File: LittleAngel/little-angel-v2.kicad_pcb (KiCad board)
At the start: 2 copper layers, 55.5 x 100 mm, 59 parts, among them J1 IN, J2 V+ GND, J3 V+ GND, J4 OUT, Q1 2N3904, SW1 SW_3PDT, U1 NE5532, U2 L78L05_TO92, U3 PT2399

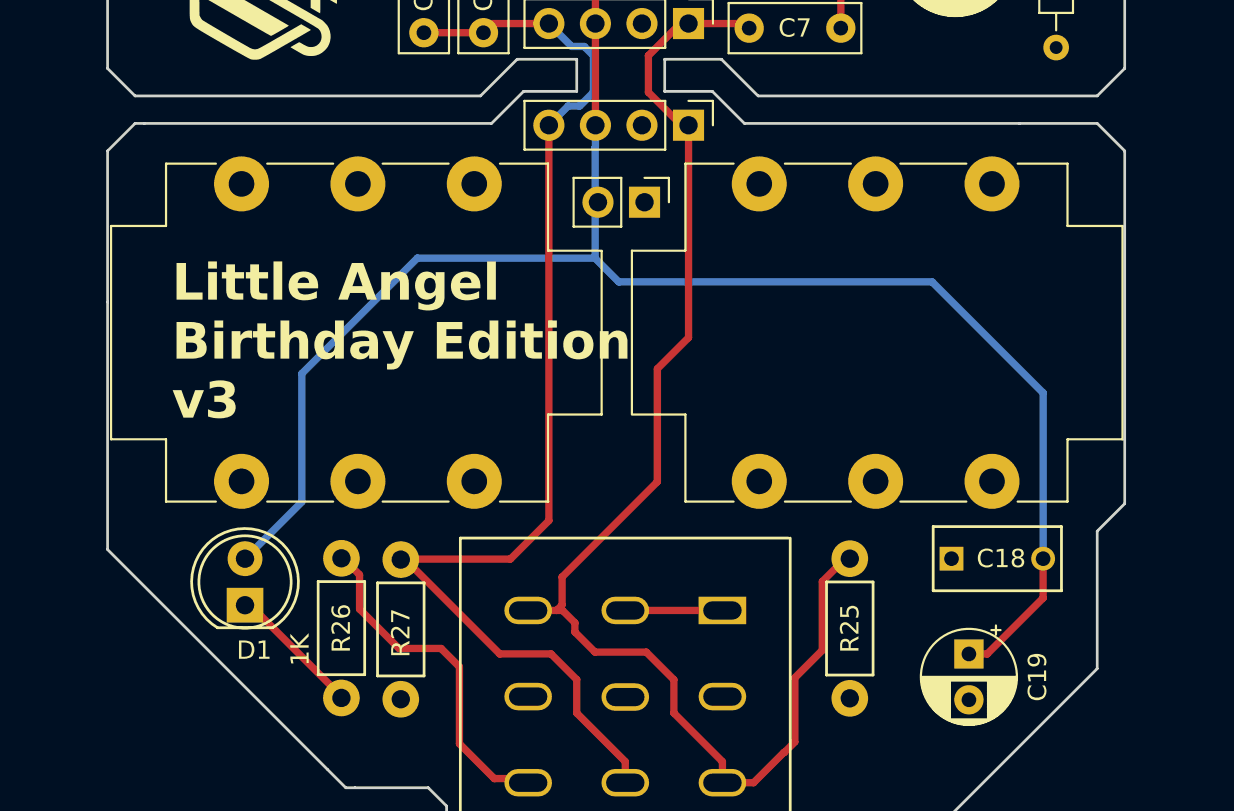
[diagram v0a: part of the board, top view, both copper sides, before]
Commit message: WIP
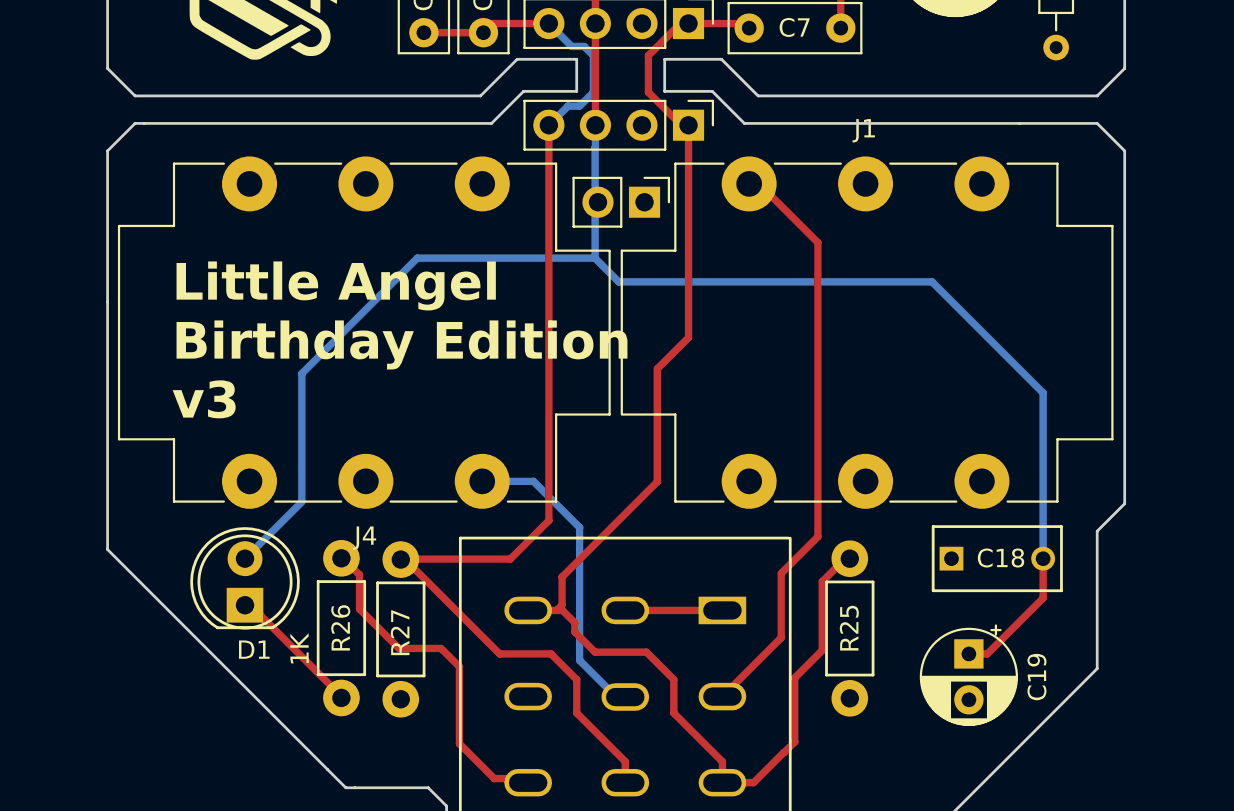
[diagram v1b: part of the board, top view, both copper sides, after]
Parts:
- J1: value IN -> NMJ6HCD2; footprint Pedal-Components:Jack_6.35mm_Neutrik_NMJ6HCD2_Horizontal -> Connector_Audio:Jack_6.35mm_Neutrik_NMJ6HCD2_Horizontal
- J4: value OUT -> NMJ6HCD2; footprint Pedal-Components:Jack_6.35mm_Neutrik_NMJ6HCD2_Horizontal -> Connector_Audio:Jack_6.35mm_Neutrik_NMJ6HCD2_Horizontal
- moved J1 0.55 mm to (150.0, 114.5)
- moved J4 0.44 mm to (135.4, 130.8)
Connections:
- J1 pad R: (no net) -> unconnected-(J1-PadR)
- J1 pad RN: (no net) -> unconnected-(J1-PadRN)
- J1 pad S: (no net) -> GND
- J1 pad SN: (no net) -> unconnected-(J1-PadSN)
- J1 pad T: (no net) -> Net-(SW1A-B)
- J1 pad TN: (no net) -> GND
- J4 pad R: (no net) -> unconnected-(J4-PadR)
- J4 pad RN: (no net) -> unconnected-(J4-PadRN)
- J4 pad S: (no net) -> GND
- J4 pad SN: (no net) -> unconnected-(J4-PadSN)
- J4 pad T: (no net) -> Net-(SW1B-B)
- J4 pad TN: (no net) -> unconnected-(J4-PadTN)
- SW1 pad 4: Net-(J1-T) -> Net-(SW1A-B)
- SW1 pad 5: Net-(J4-T) -> Net-(SW1B-B)
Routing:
- net Net-(SW1A-B): track 0.00 -> 31.5 mm
- net Net-(SW1B-B): track 0.00 -> 17.4 mm
